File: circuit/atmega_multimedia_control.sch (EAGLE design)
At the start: 4 parts, among them IC1 MEGA8-P

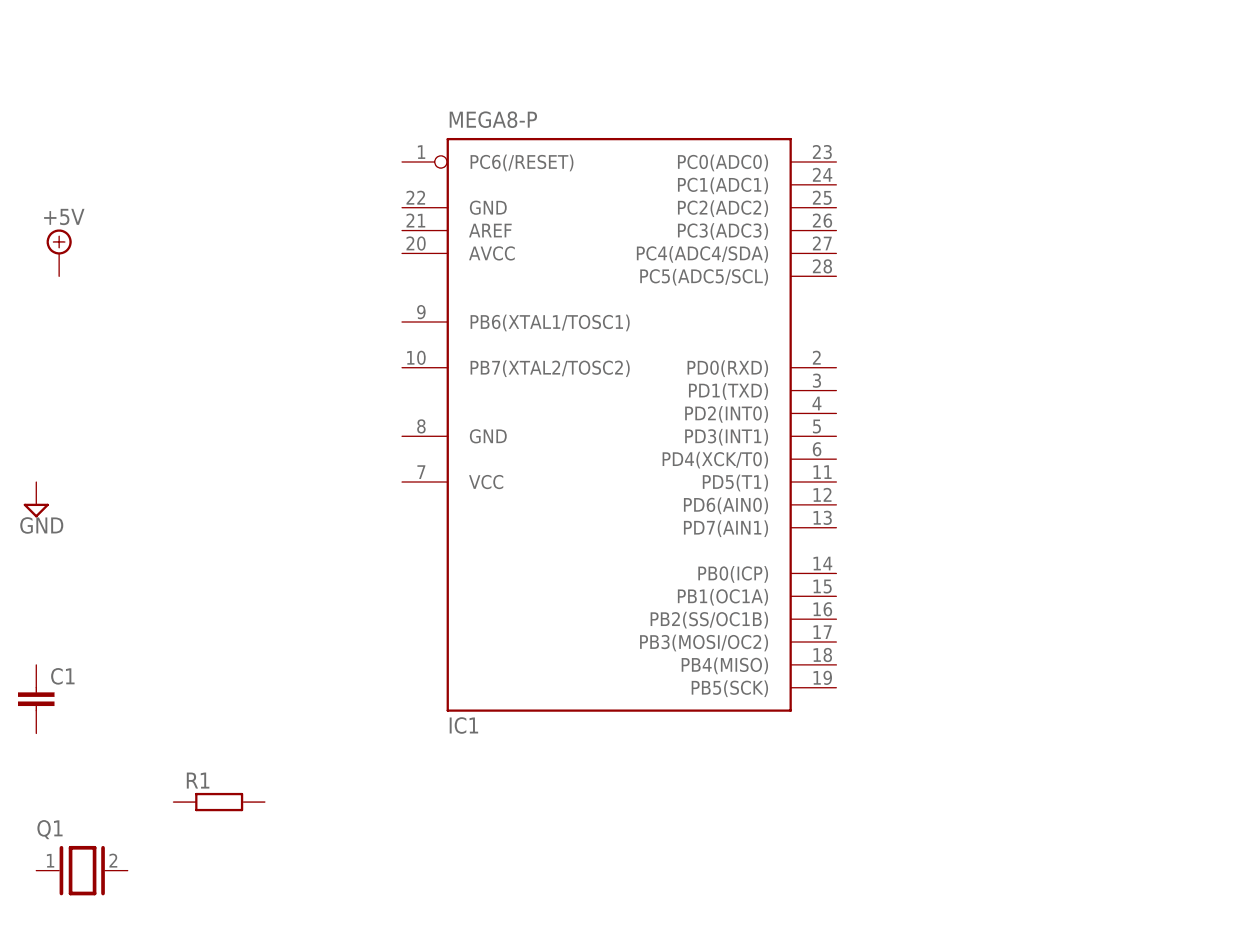
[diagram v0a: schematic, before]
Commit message: updated circuit
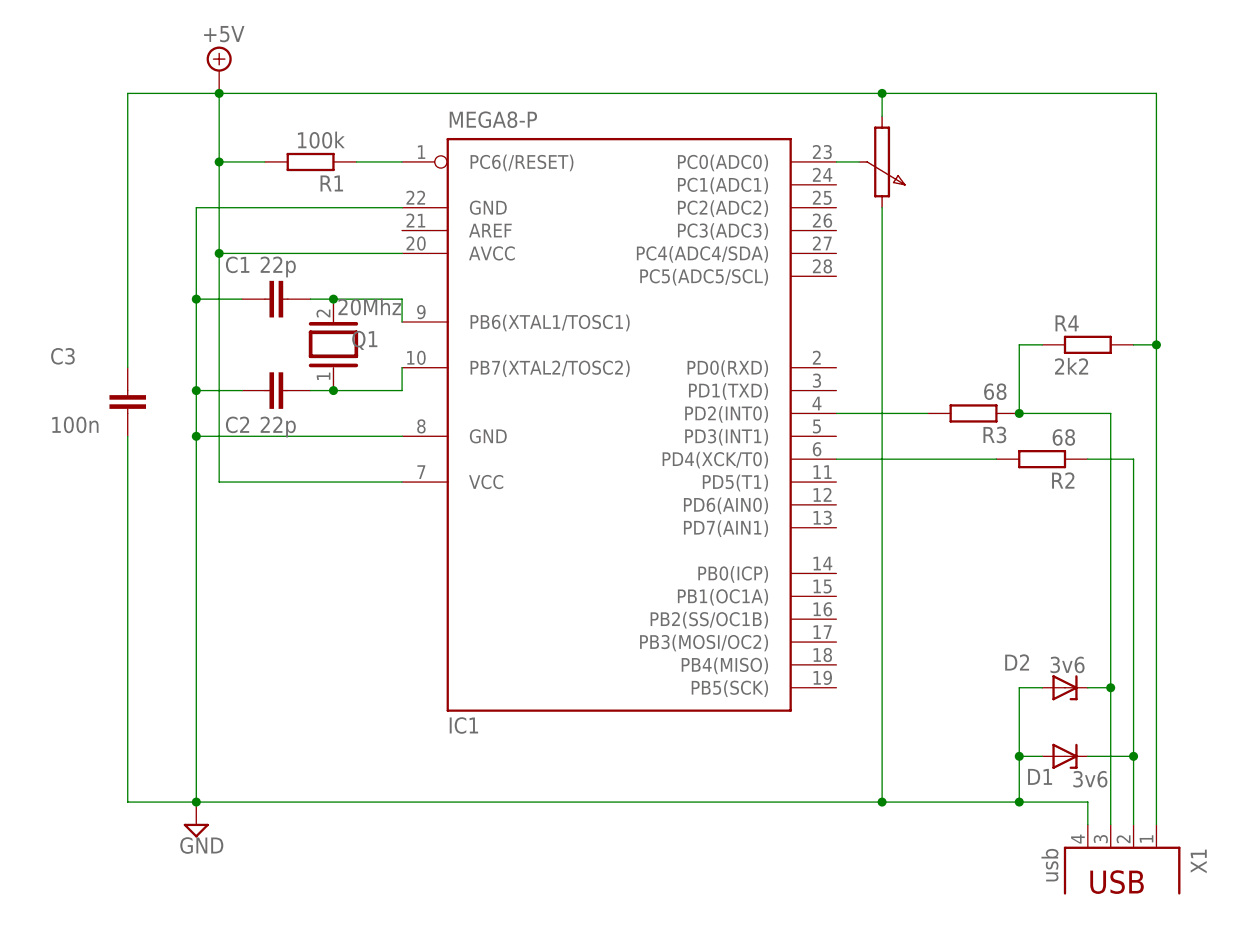
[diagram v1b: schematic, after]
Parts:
- added C2: 22p, rcl:C-EU025-025X050
- added C3: 100n, rcl:C-EU025-025X050
- added D1, D2: 3v6, diode:ZENER-DIODEDO34-7
- added R2, R3: 68, rcl:R-EU_0204/7
- added R4: 2k2, rcl:R-EU_0204/7
- added X1: usb, con-berg:PN61729
- C1: value (none) -> 22p
- Q1: value (none) -> 20Mhz
- R1: value (none) -> 100k
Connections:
- new net +5V: C3.2, IC1.AVCC, IC1.VCC@1, R1.2, R4.2, X1.1
- new net GND: C1.1, C2.1, C3.1, D1.A, D2.A, IC1.GND, IC1.GND@1, X1.4
- new net N$1: IC1.PC6(/RESET), R1.1
- new net N$2: C1.2, IC1.PB6(XTAL1/TOSC1), Q1.2
- new net N$3: C2.2, IC1.PB7(XTAL2/TOSC2), Q1.1
- new net N$4: IC1.PD4(XCK/T0), R2.2
- new net N$5: D2.C, R3.1, R4.1, X1.3
- new net N$6: D1.C, R2.1, X1.2
- new net N$7: IC1.PD2(INT0), R3.2
- new net N$8: IC1.PC0(ADC0)
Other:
- moved on the sheet: C1, Q1, R1
